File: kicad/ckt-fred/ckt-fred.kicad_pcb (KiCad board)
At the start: 2 copper layers, 73.7 x 38.1 mm, 41 parts, among them J1 Screw_Terminal_01x02, J2 AVR-ISP, J3 8P8C, J4 8P8C, J5 Screw_Terminal_01x02, SW1 FSM4JSMATR, T1 PE-51687, U1 AP7381-33Y, U2 INA180A4, U3 ATtiny85-20S, U4 TLP241A

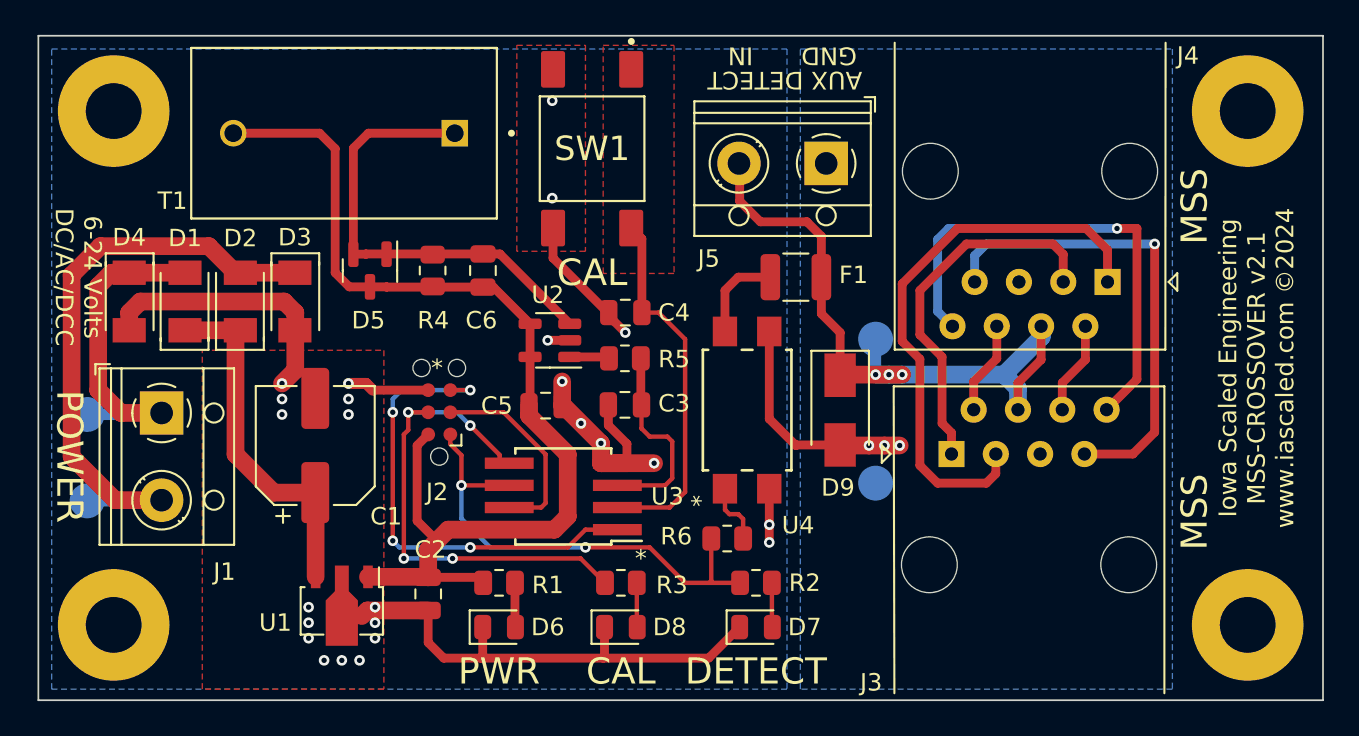
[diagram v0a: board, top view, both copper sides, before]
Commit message: Start of FRED PCB
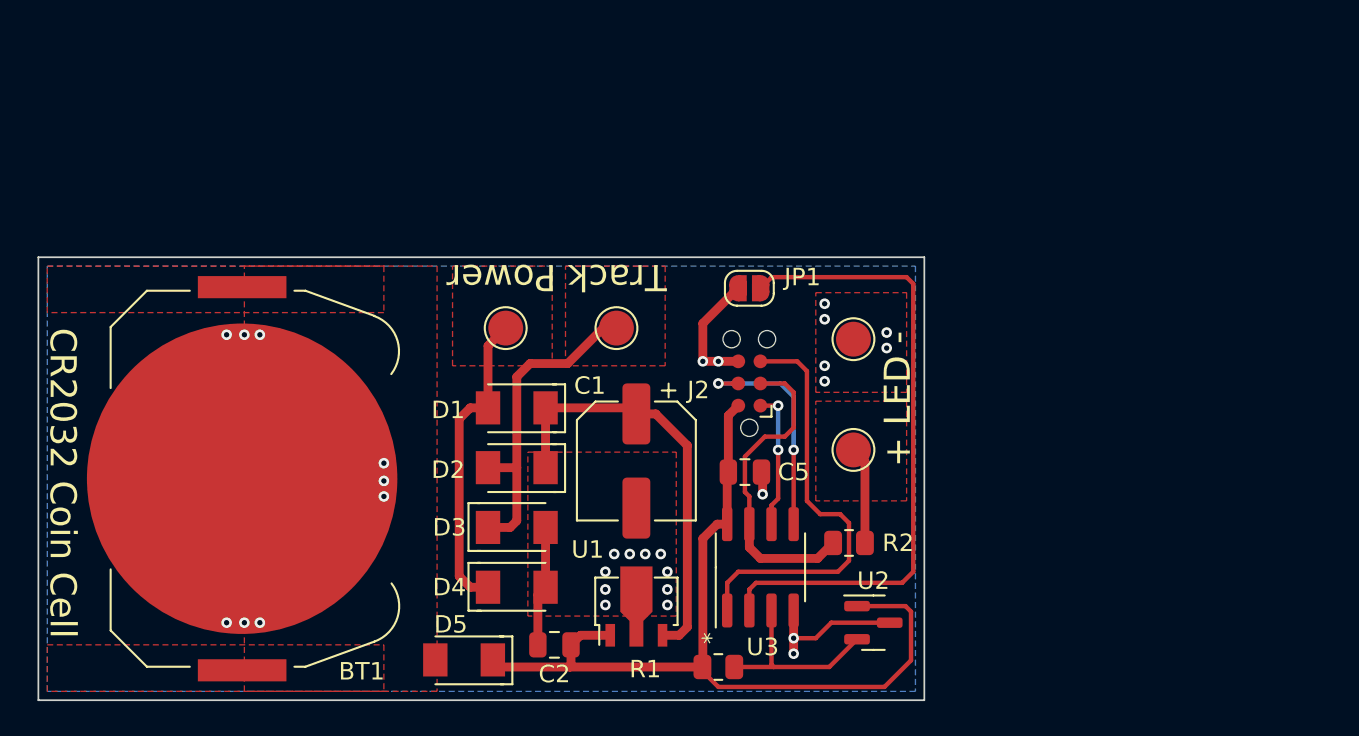
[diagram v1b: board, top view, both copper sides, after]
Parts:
- removed C3: 1uF, Capacitor_SMD:C_0805_2012Metric
- removed C4, C6: 0.1uF, Capacitor_SMD:C_0805_2012Metric
- removed D6: GREEN LED, LED_SMD:LED_0805_2012Metric
- removed D7: RED LED, LED_SMD:LED_0805_2012Metric
- removed D8: AMBER LED, LED_SMD:LED_0805_2012Metric
- removed D9: SMAJ18A-TP, Diode_SMD:D_SMA
- removed F1: 1210L020WR, Resistor_SMD:R_1210_3225Metric
- removed H1, H2, H3, H4: MountingHole, MountingHole:MountingHole_3.2mm_M3_Pad
- removed J1, J5: Screw_Terminal_01x02, TerminalBlock_RND:TerminalBlock_RND_205-00012_1x02_P5.00mm_Horizontal
- removed J3, J4: 8P8C, Connector_RJ:RJ45_Amphenol_54602-x08_Horizontal
- removed R3: 1k, Resistor_SMD:R_0805_2012Metric
- removed R4: 510, Resistor_SMD:R_0805_2012Metric
- removed R5: 100k, Resistor_SMD:R_0805_2012Metric
- removed R6: 330, Resistor_SMD:R_0805_2012Metric
- removed SW1: FSM4JSMATR, ISE_Generic:TE_FSM4JSMA
- removed T1: PE-51687, ISE_Generic:XFMR_PE-51687
- removed U4: TLP241A, ISE_UltraLibrarian:11-5B201S_TOS
- added BT1: Battery_Cell, Battery:BatteryHolder_Keystone_3034_1x20mm, F.Cu at (37.1, 179.1)
- added JP1: SolderJumper_2_Open, Jumper:SolderJumper-2_P1.3mm_Open_RoundedPad1.0x1.5mm, F.Cu at (66.2, 168.1)
- D5: value BAV99 -> BAT43W; footprint Package_TO_SOT_SMD:SOT-23 -> ISE_Generic:SOD-123T
- R1: value 1k -> 100k
- R2: value 1k -> 330
- TP1, TP2, TP3, TP4: moved to F.Cu
- U2: value INA180A4 -> DRV5032; footprint Package_TO_SOT_SMD:SOT-23-5 -> Package_TO_SOT_SMD:SOT-23
- U3: value ATtiny85-20S -> ATtiny13-20SS; footprint ISE_Generic:ATMEL_SO8_DUAL -> Package_SO:SOIC-8_3.9x4.9mm_P1.27mm
- moved TP2 31.9 mm to (58.5, 170.4), turned to 0 degrees
- moved D4 27.6 mm to (52.8, 185.3), turned to 0 degrees
- moved U2 24.6 mm to (73.3, 187.3), turned to 0 degrees
- moved TP1 24.5 mm to (52.2, 170.4), turned to 0 degrees
- moved D5 23.0 mm to (49.8, 189.5), turned to 180 degrees
- moved D1 20.0 mm to (52.8, 175.0), turned to 180 degrees
- moved D2 18.5 mm to (52.8, 178.4), turned to 180 degrees
- moved C1 18.4 mm to (59.7, 178.1), turned to -90 degrees
- moved D3 18.2 mm to (52.8, 181.9), turned to 0 degrees
- moved J2 17.9 mm to (66.2, 173.6)
- moved U1 16.9 mm to (59.7, 186.4), turned to 90 degrees
- moved R1 13.5 mm to (64.4, 189.9), turned to 0 degrees
- moved C5 12.0 mm to (65.9, 178.7)
- moved U3 12.0 mm to (66.8, 184.2), turned to 90 degrees
- moved C2 7.81 mm to (55.0, 188.6), turned to 180 degrees
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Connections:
- D5 pad 1: Net-(C6-Pad1) -> +3.3V
- D5 pad 2: Net-(C6-Pad1) -> Net-(BT1-Pad1)
- R1 pad 1: Net-(D6-Pad2) -> +3.3V
- R1 pad 2: +3.3V -> Net-(U2-Pad2)
- R2 pad 1: Net-(J2-Pad1) -> Net-(J2-Pad3)
- R2 pad 2: Net-(D7-Pad2) -> Net-(R2-Pad2)
- TP3 pad 1: /MSS_OCC -> GND
- TP4 pad 1: /MSS_GND -> Net-(R2-Pad2)
- U2 pad 1: Net-(R5-Pad2) -> +3.3V
- U2 pad 2: GND -> Net-(U2-Pad2)
- U2 pad 3: Net-(C6-Pad1) -> GND
- U3 pad 2: /~{CAL_SW} -> Net-(U3-Pad2)
- U3 pad 3: /DCC_CURRENT -> Net-(U2-Pad2)
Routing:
- net GND: track 74.5 -> 23.9 mm, vias 25 -> 30
- net /MSS_OCC: track 40.6 -> 0.00 mm, vias 3 -> 0
- net Net-(U3-Pad2): track 0.00 -> 36.7 mm
- net Net-(J3-Pad3): track 32.4 -> 0.00 mm
- net Net-(J3-Pad8): track 28.1 -> 0.00 mm, vias 1 -> 0
- net Net-(J3-Pad7): track 27.4 -> 0.00 mm, vias 1 -> 0
- net Net-(C6-Pad1): track 26.1 -> 0.00 mm
- net Net-(J3-Pad1): track 21.3 -> 0.00 mm
- net /~{CAL_SW}: track 20.7 -> 0.00 mm
- net Net-(J2-Pad1): track 27.4 -> 7.97 mm
- net Net-(D2-Pad2): track 34.7 -> 18.6 mm
- net Net-(J2-Pad4): track 28.5 -> 13.1 mm, vias 4 -> 2
- net /MSS_GND: track 13.2 -> 0.00 mm, vias 3 -> 0
- net Net-(U2-Pad2): track 0.00 -> 11.0 mm
- net +3.3V: track 61.8 -> 50.8 mm
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- added copper zone on F.Cu, net Net-(BT1-Pad1)
- added copper zone on F.Cu, net Net-(D1-Pad2)
- added copper zone on F.Cu, net Net-(D2-Pad2)
- added copper zone on F.Cu, net Net-(R2-Pad2)
- removed copper zone on B.Cu, net /MSS_GND
- removed copper zone on F.Cu, net /~{CAL_SW}
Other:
- board size 73.7 x 38.1 mm -> 50.8 x 25.4 mm
- board text added: "+ LED -"
- board text added: "CR2032 Coin Cell"
- board text added: "Iowa Scaled Engineering CKT-FRED v1.0 CC BY-SA ©2024 www.iascaled.com"
- board text added: "Track Power"
- board text removed: "6-24 Volts DC/AC/DCC"
- board text removed: "AUX DETECT"
- board text removed: "CAL"
- board text removed: "DETECT"
- board text removed: "GND"
- board text removed: "IN"
- board text removed: "Iowa Scaled Engineering MSS-CROSSOVER v2.1 www.iascaled.com ©2024"
- board text removed: "MSS"
- board text removed: "POWER"
- board text removed: "PWR"
